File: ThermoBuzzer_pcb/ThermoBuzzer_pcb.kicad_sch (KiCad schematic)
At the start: 8 parts, among them SW2 SW_Push

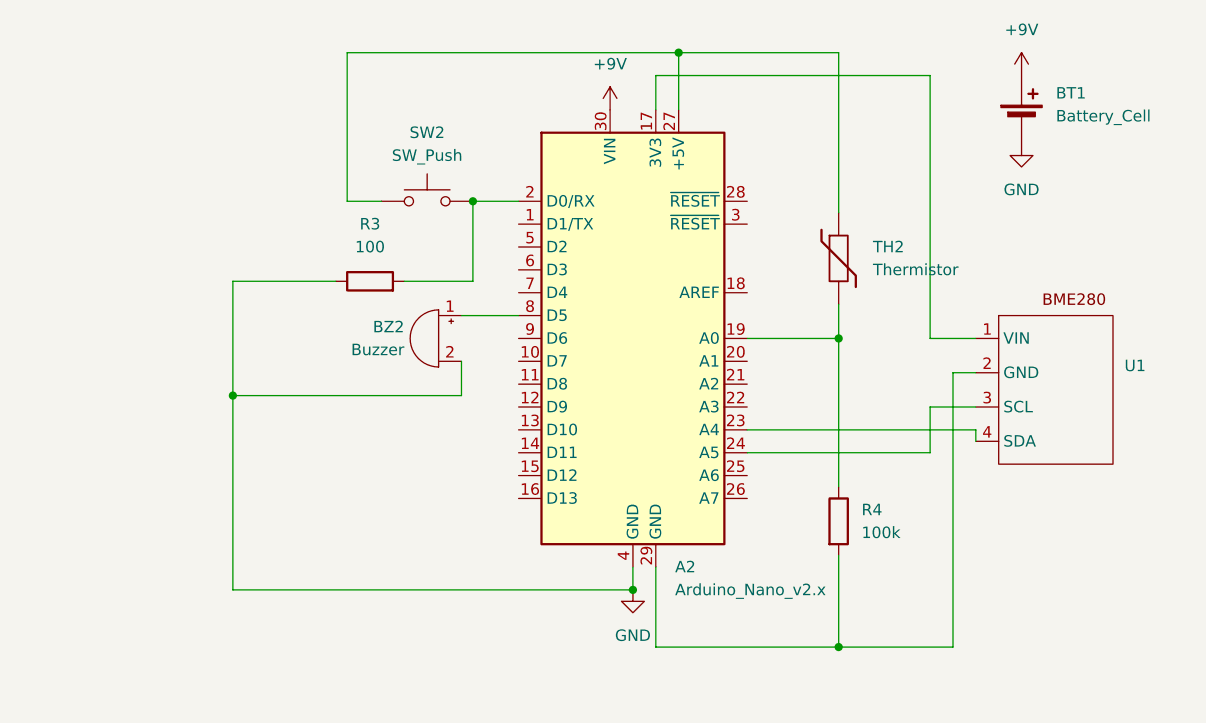
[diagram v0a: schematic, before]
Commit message: 4.15
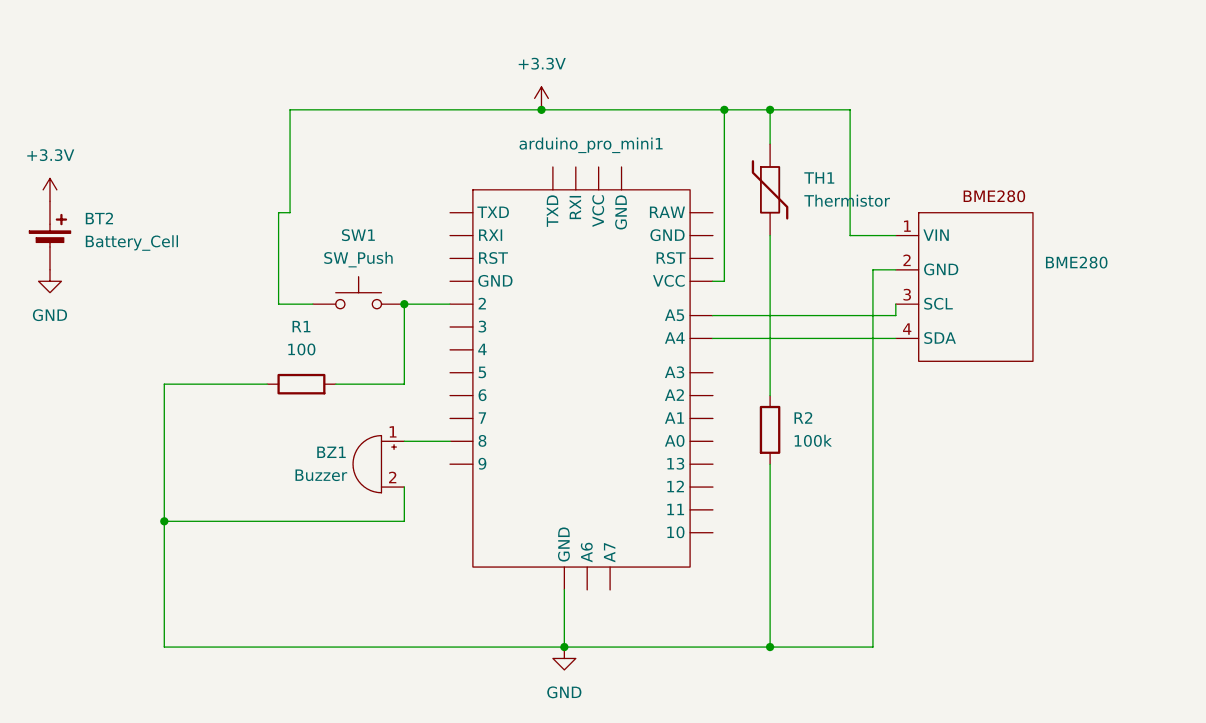
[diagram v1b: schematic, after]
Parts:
- removed A2: Arduino_Nano_v2.x, Module:Arduino_Nano, symbol MCU_Module:Arduino_Nano_v2.x
- removed BT1: Battery_Cell, Resistor_THT:R_Axial_DIN0204_L3.6mm_D1.6mm_P1.90mm_Vertical, symbol Device:Battery_Cell
- removed BZ2: Buzzer, symbol Device:Buzzer
- removed R3: 100, Resistor_THT:R_Axial_DIN0207_L6.3mm_D2.5mm_P7.62mm_Horizontal, symbol Device:R
- removed R4: 100k, Resistor_THT:R_Axial_DIN0207_L6.3mm_D2.5mm_P7.62mm_Horizontal, symbol Device:R
- removed SW2: SW_Push, symbol Switch:SW_Push
- removed TH2: Thermistor, symbol Device:Thermistor
- removed U1: ~, symbol thermosensor:BME280_new
- added BME280: ~, symbol thermosensor:BME280_new
- added BT2: Battery_Cell, Resistor_THT:R_Axial_DIN0204_L3.6mm_D1.6mm_P1.90mm_Vertical, symbol Device:Battery_Cell
- added BZ1: Buzzer, symbol Device:Buzzer
- added R1: 100, Resistor_THT:R_Axial_DIN0207_L6.3mm_D2.5mm_P7.62mm_Horizontal, symbol Device:R
- added R2: 100k, Resistor_THT:R_Axial_DIN0207_L6.3mm_D2.5mm_P7.62mm_Horizontal, symbol Device:R
- added SW1: SW_Push, symbol Switch:SW_Push
- added TH1: Thermistor, symbol Device:Thermistor
- added arduino_pro_mini1: ~, symbol thermosensor:Arduino_pro_mini
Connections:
- net GND: now also BME280.2 (GND), BT2.2 (-), BZ1.2 (-), R1.1, R2.2, arduino_pro_mini1. (10)
- new net: R1.2, SW1.2, arduino_pro_mini1. (10)
- new net: BZ1.1 (+), arduino_pro_mini1. (10)
- new net: BME280.3 (SCL), arduino_pro_mini1. (10)
- new net: BME280.4 (SDA), arduino_pro_mini1. (10)
- new net: R2.1, TH1.2
- new net +3.3V: BME280.1 (VIN), BT2.1 (+), SW1.1, TH1.1, arduino_pro_mini1. (10)

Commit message: 4.16
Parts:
- BME280: footprint (none) -> custom_footprints:AHT20+BMP280
- BZ1: footprint (none) -> Buzzer_Beeper:Buzzer_12x9.5RM7.6
- SW1: footprint (none) -> Button_Switch_THT:SW_PUSH_6mm
- TH1: footprint (none) -> Resistor_THT:R_Axial_DIN0207_L6.3mm_D2.5mm_P7.62mm_Horizontal
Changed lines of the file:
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@@
 			)
 		)
-		(property "Footprint" ""
+		(property "Footprint" "Buzzer_Beeper:Buzzer_12x9.5RM7.6"
 			(at 102.235 109.22 90)
 			(effects
@@
 			)
 		)
-		(property "Footprint" ""
+		(property "Footprint" "custom_footprints:AHT20+BMP280"
 			(at 175.26 83.82 0)
 			(effects
@@
 			)
 		)
-		(property "Footprint" ""
+		(property "Footprint" "Button_Switch_THT:SW_PUSH_6mm"
 			(at 99.06 88.9 0)
 			(effects
@@
 			)
 		)
-		(property "Footprint" ""
+		(property "Footprint" "Resistor_THT:R_Axial_DIN0207_L6.3mm_D2.5mm_P7.62mm_Horizontal"
 			(at 144.78 81.28 0)
 			(effects

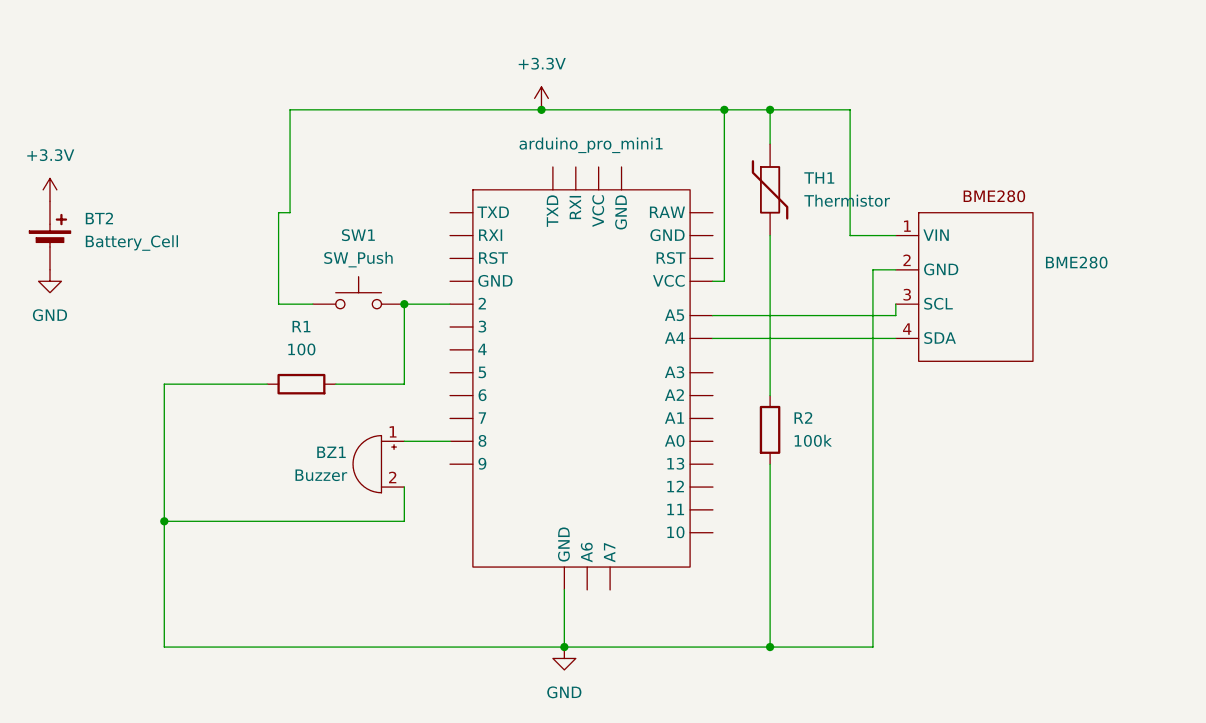
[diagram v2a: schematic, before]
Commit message: 4.18
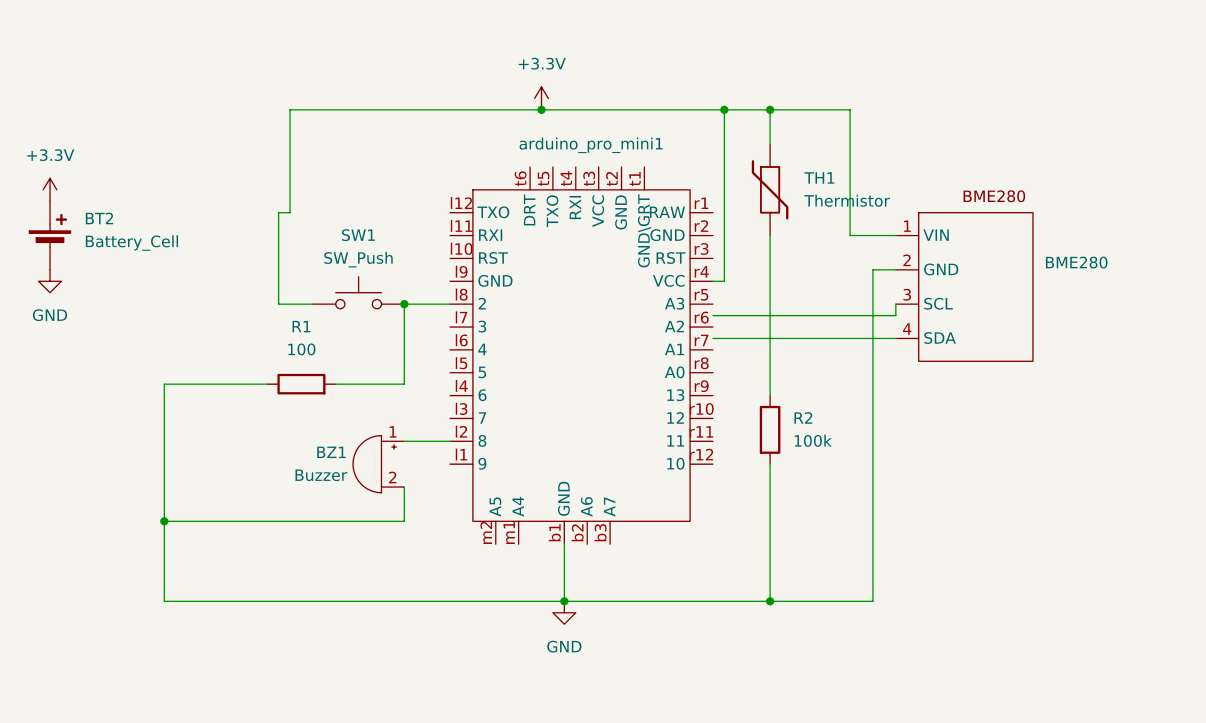
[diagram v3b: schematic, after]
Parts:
- arduino_pro_mini1: footprint (none) -> custom_footprints:arduino_pro_mini_new
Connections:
- net +3.3V: now also arduino_pro_mini1.r4 (VCC); no longer arduino_pro_mini1. (10)
- net GND: now also arduino_pro_mini1.b1 (GND); no longer arduino_pro_mini1. (10)
- net at R1.2, SW1.2: now also arduino_pro_mini1.l8 (2); no longer arduino_pro_mini1. (10)
- net at BZ1.1 (+): now also arduino_pro_mini1.l2 (8); no longer arduino_pro_mini1. (10)
- net at BME280.3 (SCL): no longer arduino_pro_mini1. (10)
- net at BME280.4 (SDA): no longer arduino_pro_mini1. (10)
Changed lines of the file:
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@@
 	)
 	(junction
-		(at 121.92 132.08)
+		(at 121.92 127)
 		(diameter 0)
 		(color 0 0 0 0)
@@
 	)
 	(junction
-		(at 144.78 132.08)
+		(at 144.78 127)
 		(diameter 0)
 		(color 0 0 0 0)
@@
 	(wire
 		(pts
-			(xy 121.92 132.08) (xy 144.78 132.08)
+			(xy 121.92 127) (xy 144.78 127)
 		)
 		(stroke
@@
 	(wire
 		(pts
-			(xy 77.47 118.11) (xy 77.47 132.08)
+			(xy 77.47 118.11) (xy 77.47 127)
 		)
 		(stroke
@@
 	(wire
 		(pts
-			(xy 156.21 90.17) (xy 156.21 132.08)
-		)
-		(stroke
-			(width 0)
-			(type default)
-		)
-	)
-	(wire
-		(pts
-			(xy 144.78 132.08) (xy 156.21 132.08)
-		)
-		(stroke
-			(width 0)
-			(type default)
-		)
-	)
-	(wire
-		(pts
-			(xy 144.78 111.76) (xy 144.78 132.08)
+			(xy 156.21 90.17) (xy 156.21 127)
+		)
+		(stroke
+			(width 0)
+			(type default)
+		)
+	)
+	(wire
+		(pts
+			(xy 144.78 127) (xy 156.21 127)
+		)
+		(stroke
+			(width 0)
+			(type default)
+		)
+	)
+	(wire
+		(pts
+			(xy 144.78 111.76) (xy 144.78 127)
 		)
 		(stroke
@@
 	(wire
 		(pts
-			(xy 77.47 132.08) (xy 121.92 132.08)
+			(xy 77.47 127) (xy 121.92 127)
 		)
 		(stroke
@@
 	(wire
 		(pts
-			(xy 121.92 125.73) (xy 121.92 132.08)
+			(xy 121.92 120.65) (xy 121.92 127)
 		)
 		(stroke
@@
 			)
 		)
-		(property "Footprint" ""
+		(property "Footprint" "custom_footprints:arduino_pro_mini_new"
 			(at 140.97 77.47 0)
 			(effects
@@
 			)
 		)
-		(pin ""
-		)
-		(pin ""
-		)
-		(pin ""
-		)
-		(pin ""
-		)
-		(pin ""
-		)
-		(pin ""
-		)
-		(pin ""
-		)
-		(pin ""
-		)
-		(pin ""
-		)
-		(pin ""
-		)
-		(pin ""
-		)
-		(pin ""
-		)
-		(pin ""
-		)
-		(pin ""
-		)
-		(pin ""
-		)
-		(pin ""
-		)
-		(pin ""
-		)
-		(pin ""
-		)
-		(pin ""
-		)
-		(pin ""
-		)
-		(pin ""
-		)
-		(pin ""
-		)
-		(pin ""
-		)
-		(pin ""
-		)
-		(pin ""
-		)
-		(pin ""
-		)
-		(pin ""
-		)
-		(pin ""
-		)
-		(pin ""
-		)
-		(pin ""
-		)
-		(pin ""
-		)
-		(pin ""
-		)
-		(pin ""
+		(pin "b3"
+		)
+		(pin "r10"
+		)
+		(pin "r11"
+		)
+		(pin "r12"
+		)
+		(pin "m1"
+		)
+		(pin "r9"
+		)
+		(pin "l3"
+		)
+		(pin "l10"
+		)
+		(pin "t5"
+		)
+		(pin "l6"
+		)
+		(pin "t6"
+		)
+		(pin "r3"
+		)
+		(pin "r2"
+		)
+		(pin "l9"
+		)
+		(pin "b2"
+		)
+		(pin "r5"
+		)
+		(pin "l12"
+		)
+		(pin "l7"
+		)
+		(pin "b1"
+		)
+		(pin "t2"
+		)
+		(pin "r7"
+		)
+		(pin "l11"
+		)
+		(pin "l4"
+		)
+		(pin "t4"
+		)
+		(pin "r6"
+		)
+		(pin "r8"
+		)
+		(pin "l8"
+		)
+		(pin "r4"
+		)
+		(pin "r1"
+		)
+		(pin "l1"
+		)
+		(pin "m2"
+		)
+		(pin "l2"
+		)
+		(pin "l5"
+		)
+		(pin "t3"
+		)
+		(pin "t1"
 		)
 		(instances
@@
 	(symbol
 		(lib_id "power:GND")
-		(at 121.92 132.08 0)
+		(at 121.92 127 0)
 		(unit 1)
 		(exclude_from_sim no)
@@
 		(fields_autoplaced yes)
 		(property "Reference" "#PWR06"
-			(at 121.92 138.43 0)
+			(at 121.92 133.35 0)
 			(effects
 				(font
@@
 		)
 		(property "Value" "GND"
-			(at 121.92 137.16 0)
+			(at 121.92 132.08 0)
 			(effects
 				(font
@@
 		)
 		(property "Footprint" ""
-			(at 121.92 132.08 0)
+			(at 121.92 127 0)
 			(effects
 				(font
@@
 		)
 		(property "Datasheet" ""
-			(at 121.92 132.08 0)
+			(at 121.92 127 0)
 			(effects
 				(font
@@
 		)
 		(property "Description" "Power symbol creates a global label with name \"GND\" , ground"
-			(at 121.92 132.08 0)
-			(effects
-				(font
+			(at 121.92 127 0)
+			(effects
+				(font
